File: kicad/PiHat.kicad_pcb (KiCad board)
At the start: 2 copper layers, 53.3 x 66.8 mm, 8 parts

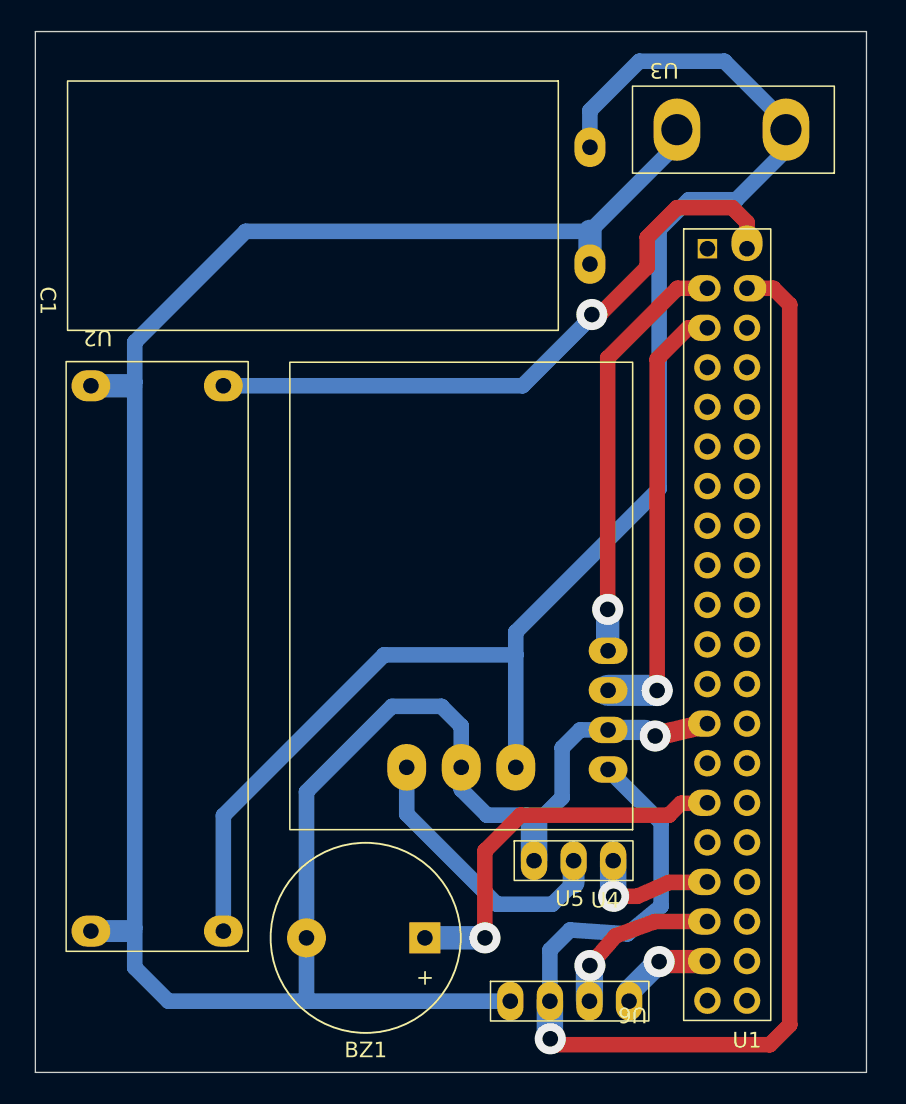
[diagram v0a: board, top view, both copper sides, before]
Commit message: Add kicad pcb
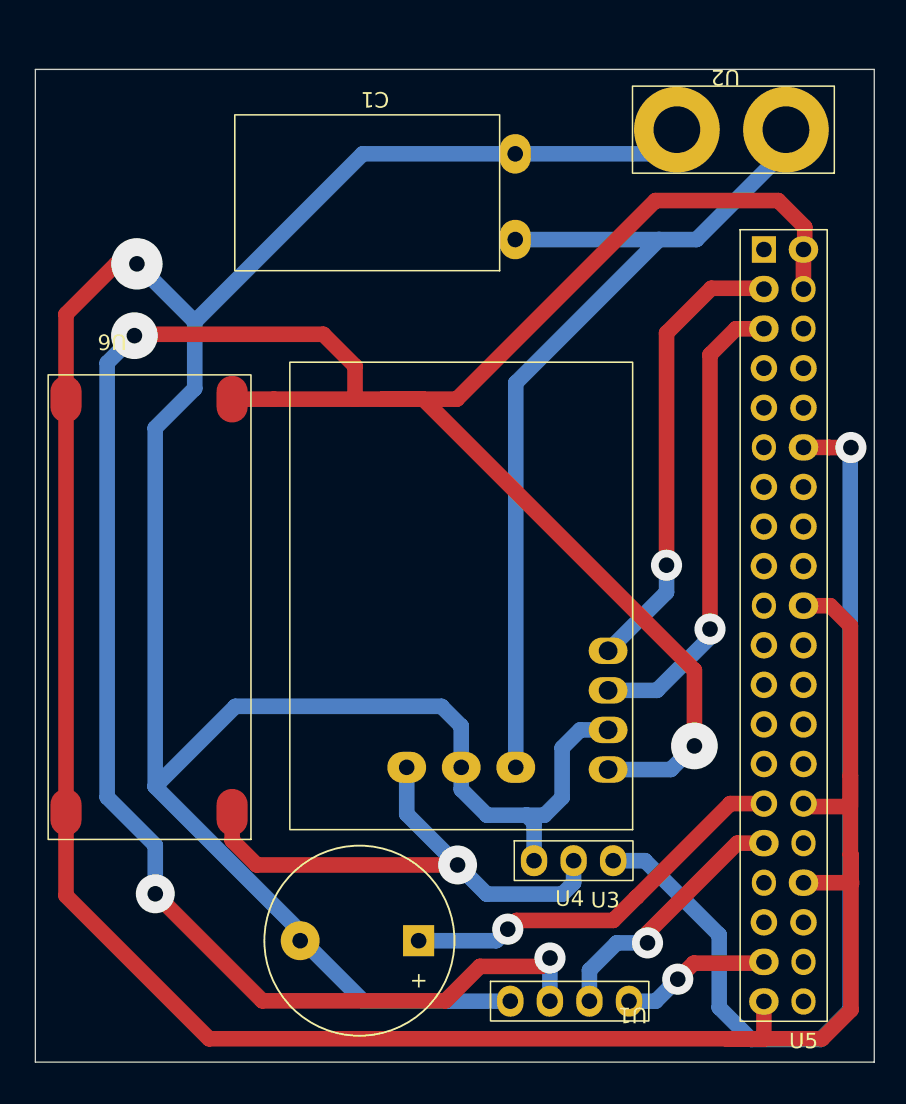
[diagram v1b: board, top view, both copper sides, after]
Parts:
- C1: value C -> 1000u; footprint Global_Custom_Library:BigCapacitor -> pi_hat:BigCapacitor
- U1: renamed from U6; value ~ -> SEN0291; footprint PiComponents:CurrentSensor -> pi_hat:CurrentSensor
- U2: renamed from U3; value ~ -> Power_Connector; footprint Global_Custom_Library:XT60 -> pi_hat:XT60
- U3: renamed from U4; value ~ -> DS3235; footprint Global_Custom_Library:Servo -> pi_hat:Servo
- U4: renamed from U5; footprint Global_Custom_Library:Encoder -> pi_hat:Encoder
- U5: renamed from U1; value ~ -> Raspberry_Pi_5; footprint Global_Custom_Library:Pi5Hat -> pi_hat:Pi5Hat
- U6: renamed from U2; value ~ -> UBEC DC/DC Converter; footprint Global_Custom_Library:5vVoltageRegulator -> pi_hat:UBEC 5V Step Down
- moved C1 13.8 mm to (147.5, 83.5), turned to 180 degrees
- moved U5 3.63 mm to (173.7, 103.7)
- moved U6 3.42 mm to (133.0, 110.0)
- moved BZ1 0.44 mm to (150.3, 131.5)
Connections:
- net Net-(BZ1-+) renamed /Buzzer_GPIO
- net Net-(U1-GPIO_2) renamed /I2C_SDA
- net Net-(U1-GPIO_26) renamed /ENCODER_A
- net Net-(U1-GPIO_3) renamed /I2C_SCL
- U1 pad 7: Net-(U4-Vin) -> +7.5V
- U3 pad 2: Net-(U4-Vin) -> +7.5V
- U3 pad 3: Net-(U1-GPIO_13) -> /PWM
- U4 pad 3: Net-(U1-GPIO_19) -> /ENCODER_B
- U5 pad 12: unconnected-(U1-GPIO_18-Pad12) -> /PWM
- U5 pad 14: unconnected-(U1-Ground-Pad14) -> GND
- U5 pad 2: Net-(U2-VOUT) -> +5V
- U5 pad 20: unconnected-(U1-Ground-Pad20) -> GND
- U5 pad 30: unconnected-(U1-Ground-Pad30) -> GND
- U5 pad 31: unconnected-(U1-GPIO_6-Pad31) -> /ENCODER_B
- U5 pad 33: Net-(U1-GPIO_13) -> unconnected-(U5-GPIO_13-Pad33)
- U5 pad 34: unconnected-(U1-Ground-Pad34) -> GND
- U5 pad 35: Net-(U1-GPIO_19) -> unconnected-(U5-GPIO_19-Pad35)
- U5 pad 39: unconnected-(U1-Ground-Pad39) -> GND
- U5 pad 6: unconnected-(U1-Ground-Pad6) -> GND
- U5 pad 9: unconnected-(U1-Ground-Pad9) -> GND
- U6 pad 2: Net-(U2-VOUT) -> +5V
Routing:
- net GND: track 167.9 -> 285.8 mm
- net +5V: track 89.7 -> 172.1 mm, vias 1 -> 4
- net /PWM: track 0.00 -> 62.9 mm, vias 0 -> 1
- net Net-(U2-VOUT): track 41.6 -> 0.00 mm, vias 1 -> 0
- net Net-(U4-Vin): track 18.1 -> 0.00 mm
- net /ENCODER_B: track 0.00 -> 16.9 mm, vias 0 -> 1
- net Net-(U1-GPIO_19): track 11.4 -> 0.00 mm, vias 1 -> 0
- net Net-(U1-GPIO_13): track 8.52 -> 0.00 mm, vias 1 -> 0
- net +7.5V: track 98.7 -> 93.7 mm, vias 0 -> 1
- net /ENCODER_A: track 6.45 -> 9.70 mm
- net /I2C_SDA: track 27.1 -> 29.4 mm
- net /I2C_SCL: track 28.5 -> 30.6 mm
- net /Buzzer_GPIO: track 25.0 -> 25.8 mm
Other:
- board size 53.3 x 66.8 mm -> 53.8 x 63.7 mm
